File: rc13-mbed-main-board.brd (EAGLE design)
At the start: 100 x 80 mm, 54 parts, among them IC1 MBED_MICROCONTROLLER, U1 PCA9555PW,118, X1 BALL_SENS, X2 ETH, X5 BTNS, X9 COIL

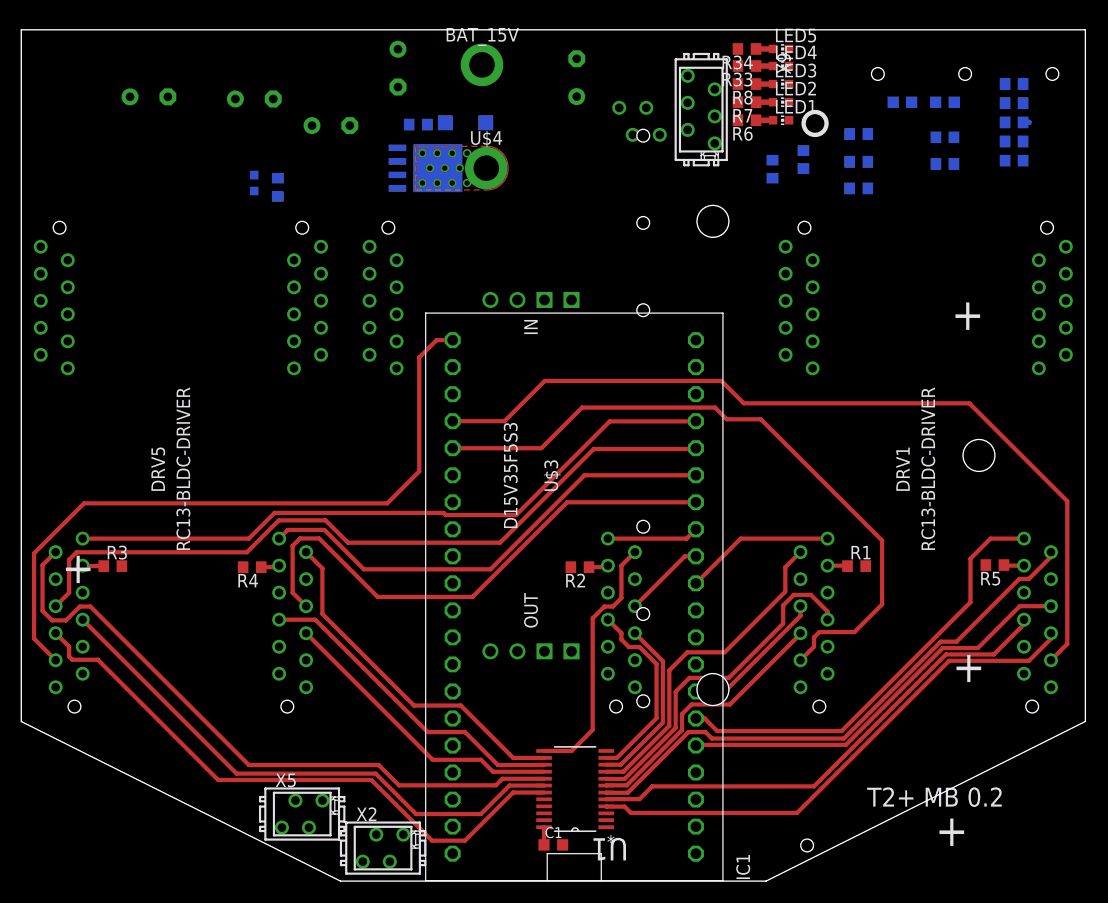
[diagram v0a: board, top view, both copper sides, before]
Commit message: Routed some board
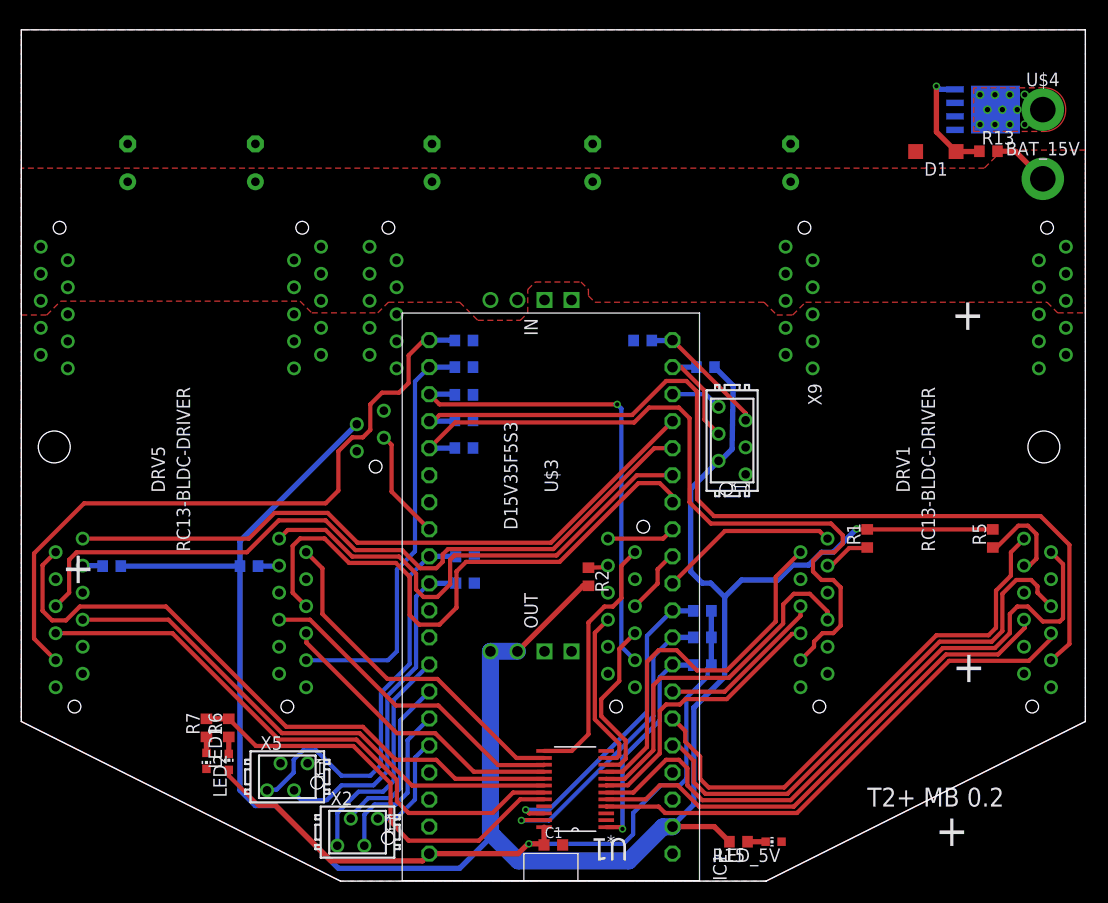
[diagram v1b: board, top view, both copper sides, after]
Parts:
- removed LED3, LED4, LED5: (no value), led:CHIP-LED0603
- removed R31, R32, R33, R34, R8: 2K2, rcl:R0603
- moved LED2 82.1 mm to (17.4, 11.3), turned to 180 degrees
- moved LED1 79.6 mm to (19.5, 11.2), turned to 0 degrees
- moved LED_5V 78.8 mm to (70.7, 3.70), flipped to the top, turned to 90 degrees
- moved R7 77.7 mm to (17.4, 14.4), turned to 90 degrees
- moved R15 75.2 mm to (67.4, 3.70), flipped to the top, turned to 180 degrees
- moved R6 75.0 mm to (19.5, 14.4), turned to 90 degrees
- moved C14 63.9 mm to (41.7, 28.0)
- moved R30 62.0 mm to (41.6, 40.7), turned to 0 degrees
- moved R28 59.7 mm to (41.6, 43.3), turned to 0 degrees
- moved C18 59.3 mm to (41.7, 30.5), turned to 180 degrees
- moved R25 57.7 mm to (41.6, 45.7), turned to 0 degrees
- moved R22 55.9 mm to (41.6, 48.3), turned to 0 degrees
- moved R19 54.4 mm to (41.6, 50.8), turned to 0 degrees
- moved BAT_15V 53.8 mm to (96.0, 66.0)
- moved R13 53.6 mm to (90.9, 68.6), flipped to the top
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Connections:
- removed net LED2: R7.2
- removed net LED3: R8.2
- removed net LED4: R33.2
- removed net LED5: R34.2, U1.20
- removed net N$10: LED_5V.A, R15.2
- removed net N$11: LED4.A, R33.1
- removed net N$12: LED5.A, R34.1
- removed net N$15: R15.1
- removed net SCL2: IC1.27, R32.1
- removed net SDA2: IC1.28, R31.1
- net +3V3: now also LED1.A; no longer R31.2, R32.2
- net +5V: now also R15.2
- net BALL: now also IC1.28
- net CHARGE: now also IC1.20; no longer IC1.19
- net GND: now also LED_5V.A; no longer LED1.C, LED3.C, LED4.C, LED5.C
- net KICK: now also IC1.19; no longer IC1.20
- net LED1: now also R7.2, U1.20
- net N$7: now also LED1.C; no longer LED1.A
- net N$9: now also LED_5V.C, R15.1; no longer LED3.A, R8.1
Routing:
- net +5V: track 0.00 -> 209.8 mm, vias 0 -> 1
- net +3V3: track 1.67 -> 71.2 mm, vias 0 -> 1
- net PWM3: track 0.57 -> 45.2 mm, vias 0 -> 1
- net LED1: track 0.00 -> 40.2 mm
- net PWM4: track 0.00 -> 39.2 mm
- net BTN2: track 0.00 -> 38.4 mm
- net BTN1: track 0.00 -> 32.2 mm
- net SCL: track 0.18 -> 29.6 mm, vias 0 -> 1
- net SDA: track 0.00 -> 28.7 mm, vias 0 -> 1
- net TD+: track 0.00 -> 22.0 mm
- net INT: track 0.06 -> 21.0 mm, vias 0 -> 1
- net TD-: track 0.00 -> 16.2 mm
- net RD+: track 0.00 -> 15.7 mm
- net CHARGE: track 0.00 -> 12.3 mm
- net TACHO2: track 38.8 -> 50.4 mm
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- added copper zone on layer 1, net +15V
- added copper zone on layer 1, net GND
- added copper zone on layer 16, net GND
